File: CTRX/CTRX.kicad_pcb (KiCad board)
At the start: 4 copper layers, 45 x 19 mm, 37 parts, among them J1 CON-SMA-EDGE-S, J3 Conn_02x05_Odd_Even, J4 USB-AM-S-X-X-TH, U1 nRF52820-QDxx, U2 NRF21540-QDAA-R7, U3 USBLC6-2SC6, U4 ME6211C33M5, Y1 32MHz

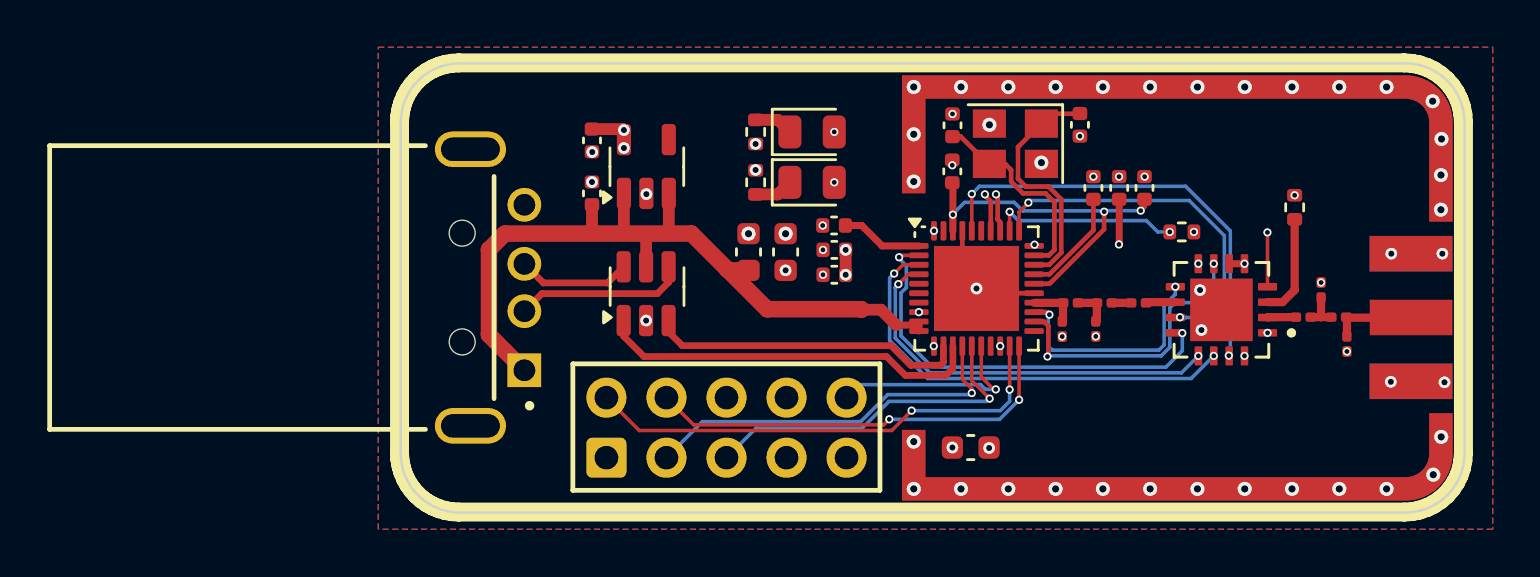
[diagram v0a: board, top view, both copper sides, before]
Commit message: via correction
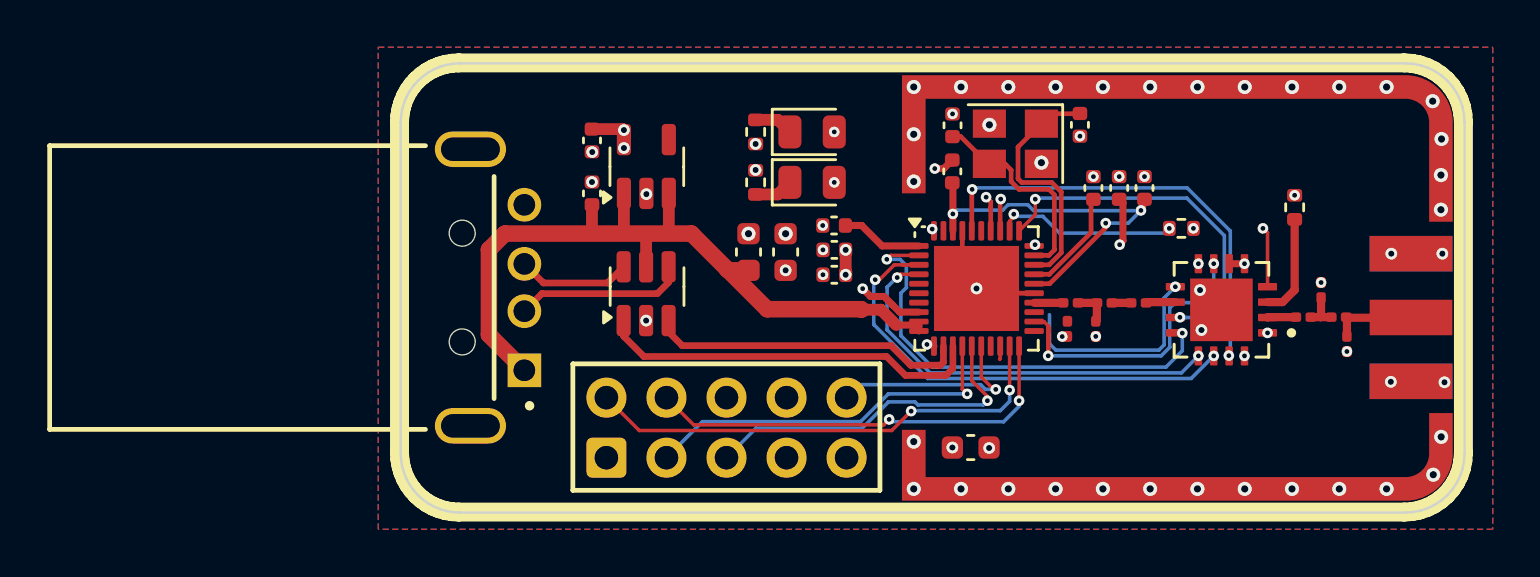
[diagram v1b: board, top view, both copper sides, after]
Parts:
- moved C2 0.22 mm to (142.7, 90.0)
- moved R1 0.15 mm to (147.5, 85.8)
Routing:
- net +3.3V: track 45.5 -> 49.0 mm, vias 11 -> 10
- net NRF_PA_TX_EN: track 10.2 -> 8.94 mm, vias 2 -> 1
- net DEC4: track 15.6 -> 16.7 mm
- net NRF_SPI0_SCK: track 17.9 -> 18.9 mm
- net NRF_SPI0_MISO: track 18.9 -> 19.9 mm
- net GND: track 5.43 -> 6.32 mm
- net Net-(U1-ANT): track 2.01 -> 1.21 mm
- net USBDEC: track 4.83 -> 5.48 mm

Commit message: CTRX Order V3 - VIA Update
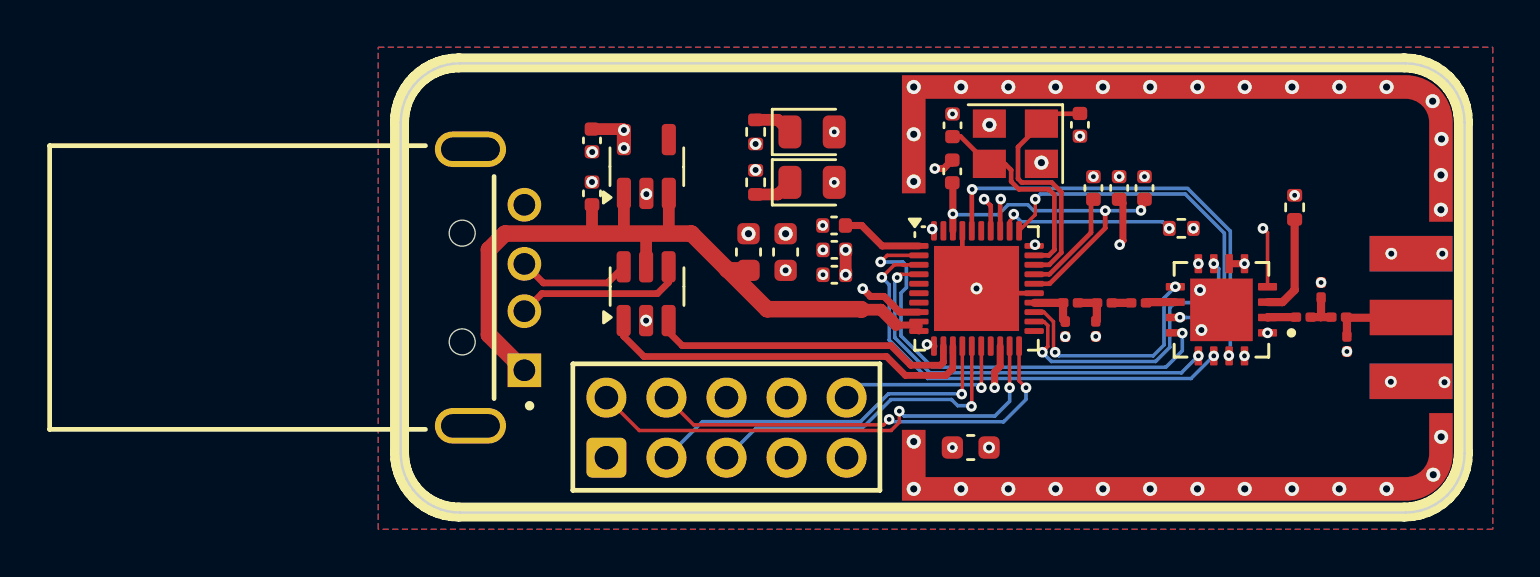
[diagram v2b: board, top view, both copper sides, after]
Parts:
- moved C2 0.09 mm to (142.6, 90.0)
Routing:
- net +3.3V: track 49.0 -> 51.1 mm, vias 10 -> 11
- net DEC4: track 16.7 -> 15.6 mm
- net NRF_NRST: track 8.76 -> 7.80 mm
- net NRF_PA_TX_EN: track 8.94 -> 9.83 mm, vias 1 -> 2
- net Net-(U1-ANT): track 1.21 -> 2.04 mm
- net P015: track 14.7 -> 14.1 mm
- net NRF_SWDIO: track 20.5 -> 21.0 mm
- net NRF_PA_RX_EN: track 12.4 -> 12.9 mm
- net NRF_SPI0_SCK: track 18.9 -> 19.4 mm
